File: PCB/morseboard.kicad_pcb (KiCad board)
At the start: 2 copper layers, 100.5 x 93 mm, 23 parts, among them J1 Conn_01x04_Socket, SW1 SW_Push, SW2 SW_Push, SW3 SW_Push, SW4 SW_Push, SW5 SW_Push, SW6 SW_Push, SW7 RotaryEncoder_Switch, U1 XIAO-RP2040-DIP

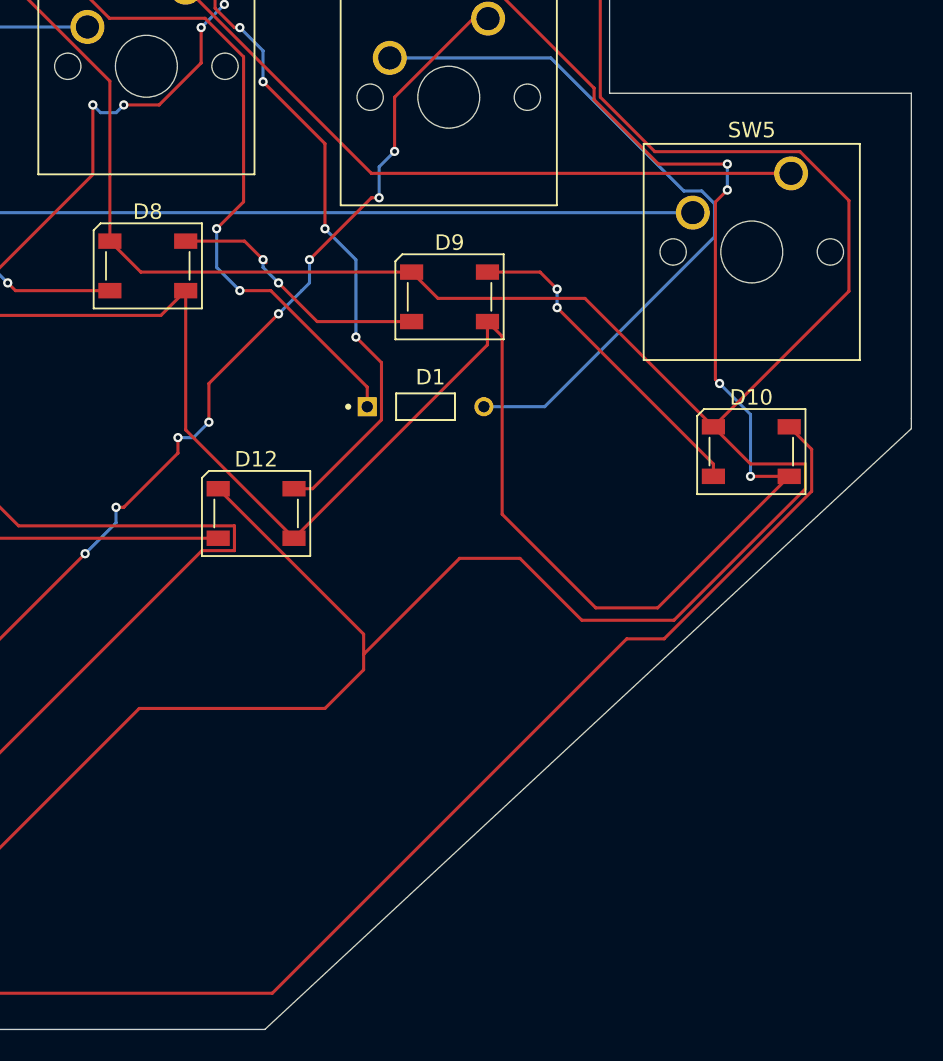
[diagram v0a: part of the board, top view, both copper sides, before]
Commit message: branding
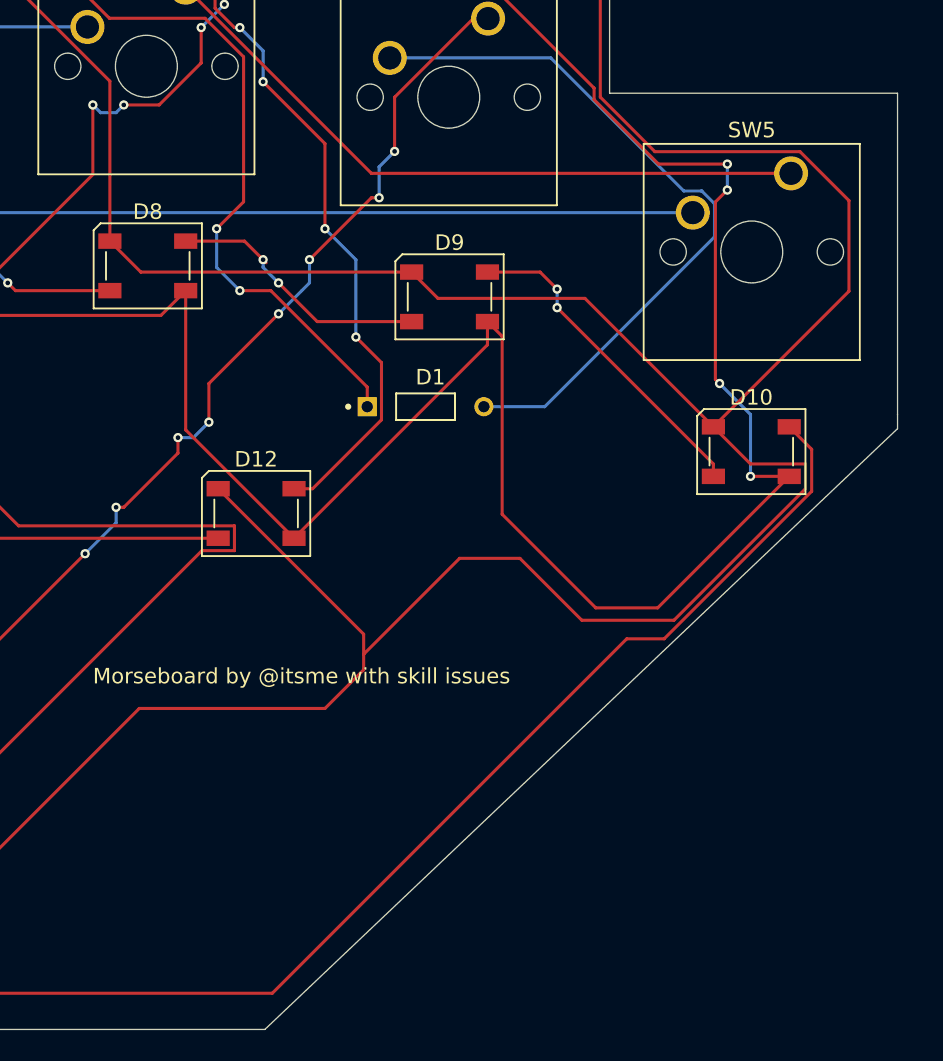
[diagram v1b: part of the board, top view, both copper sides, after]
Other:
- board size 100.5 x 93 mm -> 99.6 x 93 mm
- board text added: "Morseboard by @itsme with skill issues"
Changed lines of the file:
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@@
 			(xy 131.590454 138.243143) (xy 126.893086 112.743143) (xy 126.893086 47.743143) (xy 147.893086 47.743143)
 			(xy 147.893086 48.243143) (xy 167.393086 48.243143) (xy 167.393086 45.243143) (xy 188.393086 45.243143)
-			(xy 188.393086 47.743143) (xy 207.893086 47.743143) (xy 207.893086 77.743143) (xy 227.393086 77.743143)
-			(xy 227.393086 98.743143) (xy 227.393086 99.419909) (xy 185.615911 138.243143)
+			(xy 188.393086 47.743143) (xy 207.893086 47.743143) (xy 207.893086 77.743143) (xy 226.5 77.743143)
+			(xy 226.5 98.5) (xy 226.5 99.419909) (xy 185.615911 138.243143)
 		)
 		(stroke
@@
 		(layer "Edge.Cuts")
 	)
+	(gr_text "Morseboard by @itsme with skill issues"
+		(at 174.5 116 0)
+		(layer "F.SilkS")
+		(effects
+			(font
+				(size 1 1)
+				(thickness 0.1)
+			)
+			(justify left bottom)
+		)
+	)
 	(segment
